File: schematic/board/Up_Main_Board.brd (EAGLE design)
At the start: 79.9 x 73.5 mm, 18 parts

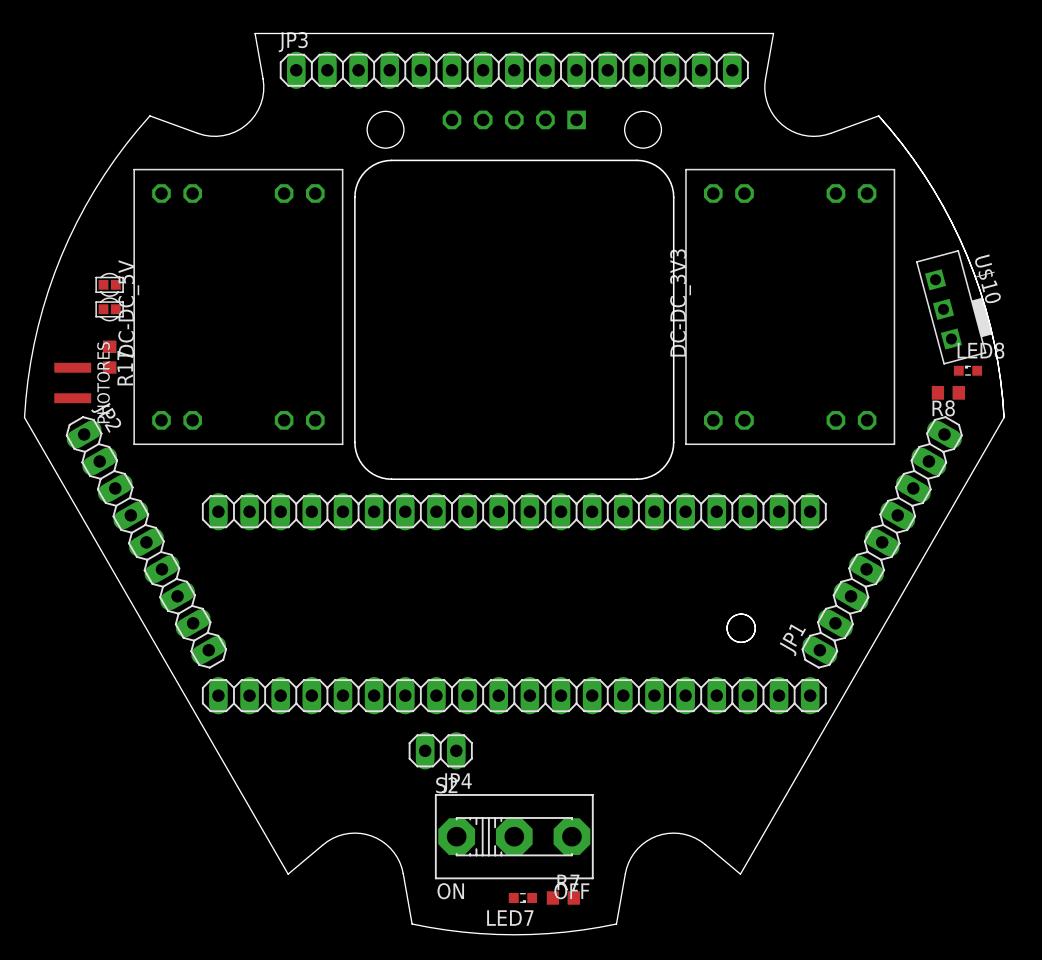
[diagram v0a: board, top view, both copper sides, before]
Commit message: Развод на плате...
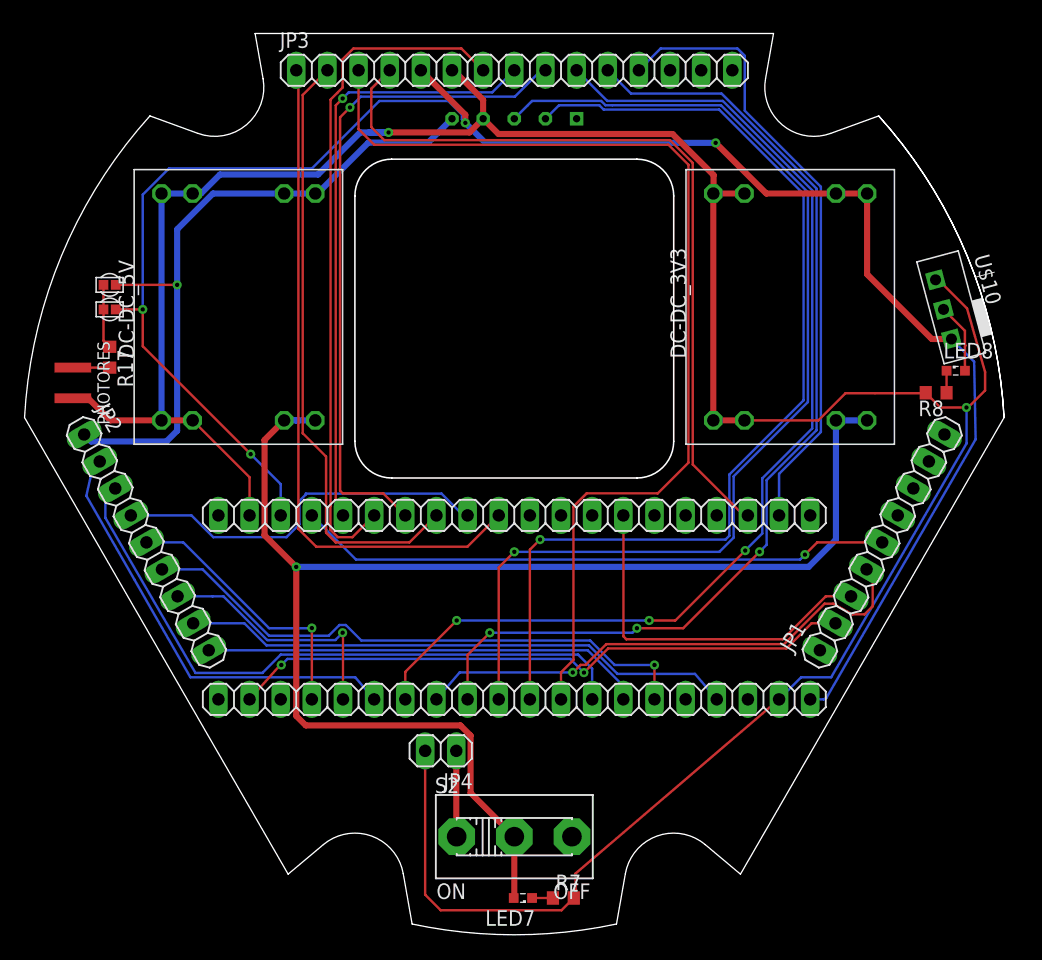
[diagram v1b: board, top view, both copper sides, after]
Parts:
- U$3: device NEON-BLADE-2024:GPS_NEO7M_W-PPS_&_ANT -> NEON-BLADE-2023:GPS_NEO7M_W-PPS_&_ANT
- moved LED8 1.00 mm to (86.0, 56.0)
- moved R8 1.00 mm to (84.4, 54.2)
- moved U$2 0.30 mm to (50.0, 36.7)
- moved U$3 0.10 mm to (50.0, 58.1)
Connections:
- removed net N$2: DC-DC_5V.P$3, DC-DC_5V.P$4
- removed net N$3: DC-DC_3V3.P$3, DC-DC_3V3.P$4
- removed net SPI4_SCK: U$2.22
- new net 4SCK: JP1.2, U$2.22
- net 4MISO: now also JP1.4
- net 4MOSI: now also JP1.3
- net 5MISO: no longer JP1.4
- net 5MOSI: no longer JP1.3
- net 5SCK: no longer JP1.2
- net GND: now also DC-DC_3V3.P$3, DC-DC_3V3.P$4, DC-DC_5V.P$3, DC-DC_5V.P$4
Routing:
- net GND: track 0.00 -> 230.6 mm, vias 0 -> 2
- net 3V3: track 0.00 -> 154.7 mm, vias 0 -> 4
- net V_BAT: track 0.00 -> 115.2 mm, vias 0 -> 1
- net GPS_TX: track 0.00 -> 89.2 mm, vias 0 -> 1
- net 5MOSI: track 0.00 -> 89.0 mm, vias 0 -> 3
- net 1MISO: track 0.00 -> 84.2 mm
- net GPS_RX: track 0.00 -> 83.8 mm, vias 0 -> 1
- net 5MISO: track 0.00 -> 83.5 mm, vias 0 -> 3
- net CS_LIS: track 0.00 -> 63.5 mm
- net CE_NRF: track 0.00 -> 55.9 mm
- net 5V: track 0.00 -> 55.8 mm, vias 0 -> 1
- net 1SCK: track 0.00 -> 55.5 mm
- net 5SCK: track 0.00 -> 54.9 mm, vias 0 -> 1
- net SDIO_DAT3: track 0.00 -> 53.3 mm
- net 4SCK: track 0.00 -> 51.4 mm, vias 0 -> 2
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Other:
- outline, holes or cut-outs redrawn
